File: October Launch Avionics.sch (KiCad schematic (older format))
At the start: 30 parts, among them IC1 MPU-6050, IC2 790, IC3 BMP384, J1 U.FL-R-SMT_01_, J2 MEM2075-00-140-01-A, U1 ESP32-WROOM-32D, U2 LM2596S-5

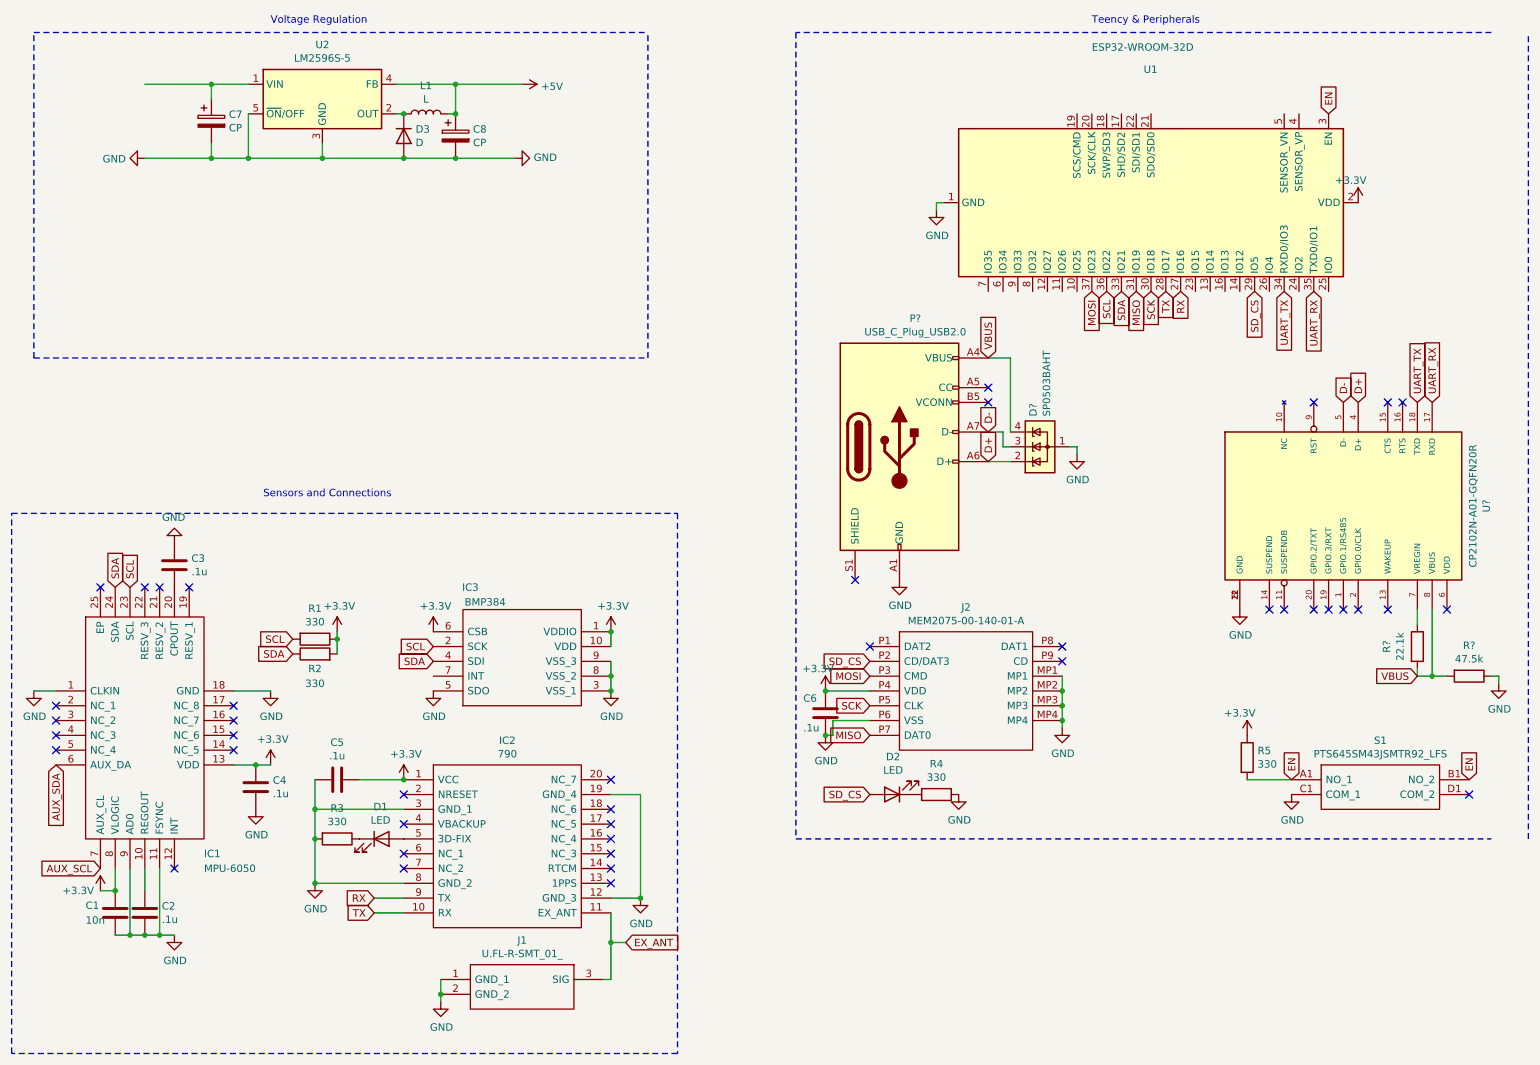
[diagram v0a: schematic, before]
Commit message: Fixed some merging weirdness?
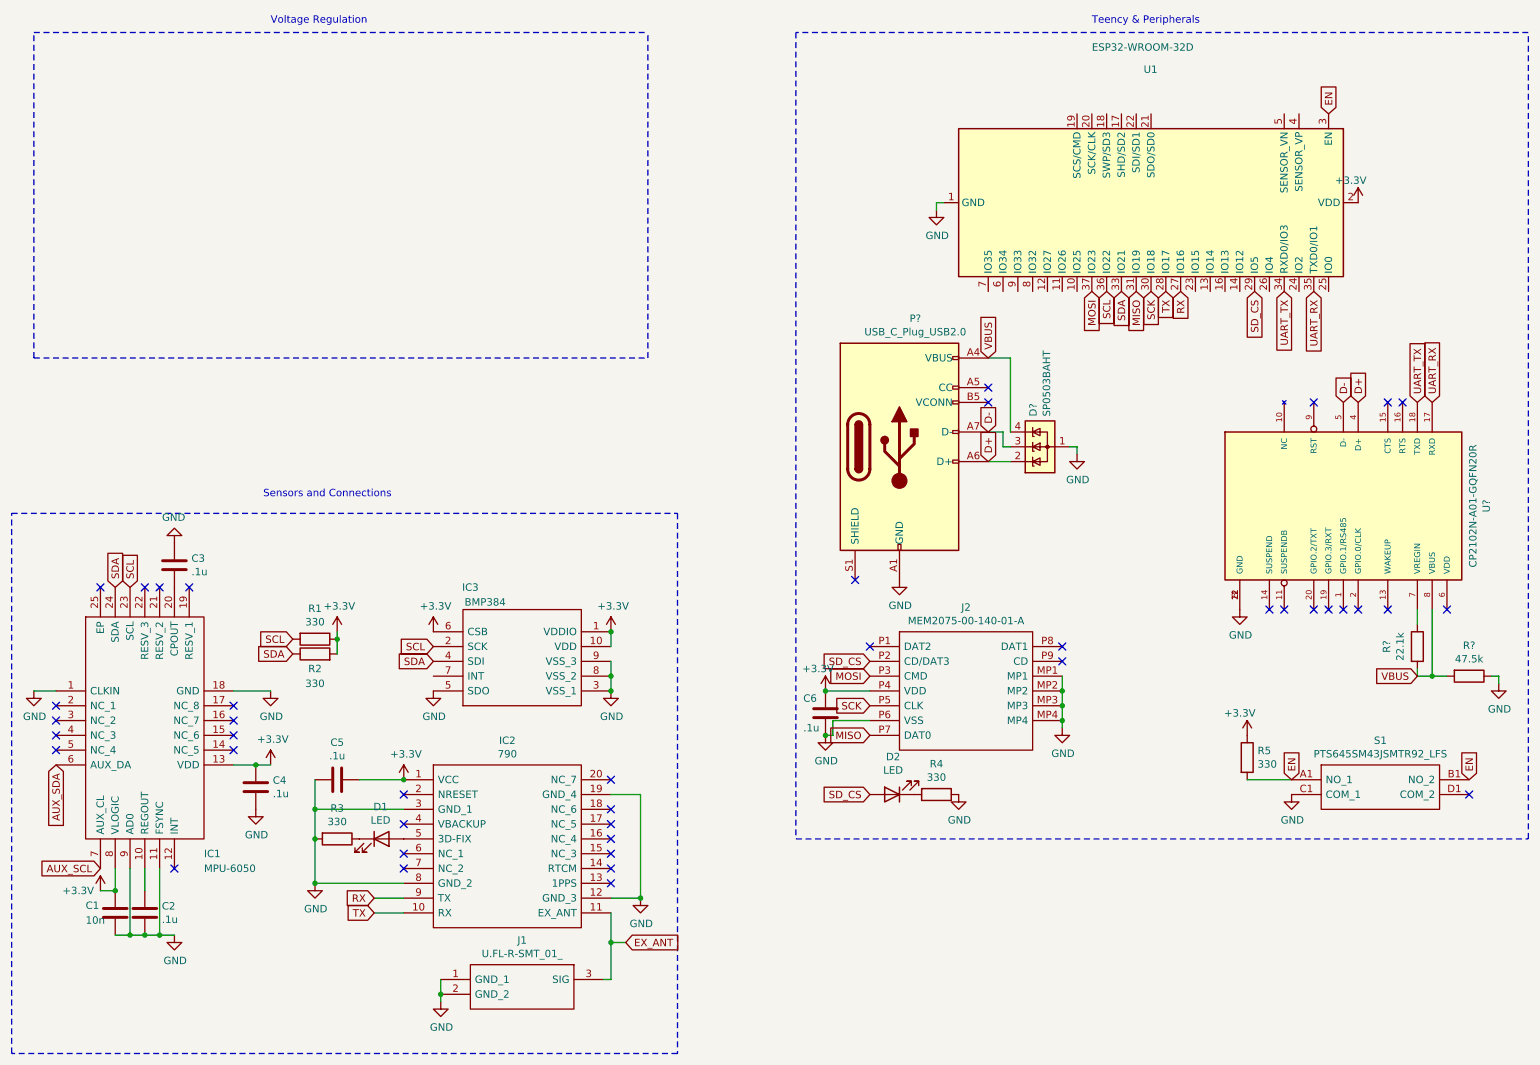
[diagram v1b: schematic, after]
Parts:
- removed C7, C8: CP, symbol Device:CP
- removed D3: D, symbol Device:D
- removed L1: L, symbol Device:L
- removed U2: LM2596S-5, Package_TO_SOT_SMD:TO-263-5_TabPin3, symbol Regulator_Switching:LM2596S-5
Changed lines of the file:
@@
 	6000 800  6000 6250
 Wire Notes Line
-	10700 800  6000 800
+	10950 800  6000 800
 Text Notes 8000 750  0    50   ~ 0
 Teency & Peripherals
@@
 	10950 6250 10950 800
 Wire Notes Line
-	6000 6250 10700 6250
+	6000 6250 10950 6250
 Text GLabel 9700 3300 1    50   Input ~ 0
 D-
@@
 Wire Wire Line
 	7450 3000 7450 3500
-$Comp
-L Regulator_Switching:LM2596S-5 U2
-U 1 1 61015F13
-P 2800 1250
-F 0 "U2" H 2800 1617 50  0000 C CNN
-F 1 "LM2596S-5" H 2800 1526 50  0000 C CNN
-F 2 "Package_TO_SOT_SMD:TO-263-5_TabPin3" H 2850 1000 50  0001 L CIN
-F 3 "http://www.ti.com/lit/ds/symlink/lm2596.pdf" H 2800 1250 50  0001 C CNN
-	1    2800 1250
-	1    0    0    -1
-$EndComp
-$Comp
-L power:+5V #PWR0107
-U 1 1 6102E3B5
-P 4150 1150
-F 0 "#PWR0107" H 4150 1000 50  0001 C CNN
-F 1 "+5V" V 4165 1278 50  0000 L CNN
-F 2 "" H 4150 1150 50  0001 C CNN
-F 3 "" H 4150 1150 50  0001 C CNN
-	1    4150 1150
-	0    1    1    0
-$EndComp
-$Comp
-L Device:L L1
-U 1 1 610792E4
-P 3500 1350
-F 0 "L1" V 3690 1350 50  0000 C CNN
-F 1 "L" V 3599 1350 50  0000 C CNN
-F 2 "" H 3500 1350 50  0001 C CNN
-F 3 "~" H 3500 1350 50  0001 C CNN
-	1    3500 1350
-	0    -1   -1   0
-$EndComp
-$Comp
-L Device:D D3
-U 1 1 61076105
-P 3350 1500
-F 0 "D3" V 3304 1580 50  0000 L CNN
-F 1 "D" V 3395 1580 50  0000 L CNN
-F 2 "" H 3350 1500 50  0001 C CNN
-F 3 "~" H 3350 1500 50  0001 C CNN
-	1    3350 1500
-	0    1    1    0
-$EndComp
-Connection ~ 3350 1650
-$Comp
-L power:GND #PWR0105
-U 1 1 61028B2E
-P 1600 1650
-F 0 "#PWR0105" H 1600 1400 50  0001 C CNN
-F 1 "GND" V 1605 1522 50  0000 R CNN
-F 2 "" H 1600 1650 50  0001 C CNN
-F 3 "" H 1600 1650 50  0001 C CNN
-	1    1600 1650
-	0    1    1    0
-$EndComp
-Wire Wire Line
-	2300 1350 2300 1650
-Connection ~ 2300 1650
-Wire Wire Line
-	2300 1650 2800 1650
-Wire Wire Line
-	2800 1550 2800 1650
-Connection ~ 2800 1650
-Wire Wire Line
-	2800 1650 3350 1650
-Wire Wire Line
-	3300 1350 3350 1350
-Connection ~ 3350 1350
-Wire Wire Line
-	3650 1350 3700 1350
-Wire Wire Line
-	3700 1350 3700 1150
-Connection ~ 3700 1150
-Wire Wire Line
-	3700 1150 3300 1150
-Wire Wire Line
-	3700 1150 4150 1150
-$Comp
-L power:GND #PWR0106
-U 1 1 610A5901
-P 4100 1650
-F 0 "#PWR0106" H 4100 1400 50  0001 C CNN
-F 1 "GND" V 4105 1522 50  0000 R CNN
-F 2 "" H 4100 1650 50  0001 C CNN
-F 3 "" H 4100 1650 50  0001 C CNN
-	1    4100 1650
-	0    -1   -1   0
-$EndComp
-$Comp
-L Device:CP C8
-U 1 1 610A7BB2
-P 3700 1500
-F 0 "C8" H 3818 1546 50  0000 L CNN
-F 1 "CP" H 3818 1455 50  0000 L CNN
-F 2 "" H 3738 1350 50  0001 C CNN
-F 3 "~" H 3700 1500 50  0001 C CNN
-	1    3700 1500
-	1    0    0    -1
-$EndComp
-Wire Wire Line
-	3350 1650 3700 1650
-Connection ~ 3700 1350
-Connection ~ 3700 1650
-Wire Wire Line
-	3700 1650 4100 1650
-$Comp
-L Device:CP C7
-U 1 1 610AC176
-P 2050 1400
-F 0 "C7" H 2168 1446 50  0000 L CNN
-F 1 "CP" H 2168 1355 50  0000 L CNN
-F 2 "" H 2088 1250 50  0001 C CNN
-F 3 "~" H 2050 1400 50  0001 C CNN
-	1    2050 1400
-	1    0    0    -1
-$EndComp
-Wire Wire Line
-	1600 1150 2050 1150
-Wire Wire Line
-	1600 1650 2050 1650
-Wire Wire Line
-	2050 1250 2050 1150
-Connection ~ 2050 1150
-Wire Wire Line
-	2050 1150 2300 1150
-Wire Wire Line
-	2050 1550 2050 1650
-Connection ~ 2050 1650
-Wire Wire Line
-	2050 1650 2300 1650
 $EndSCHEMATC
